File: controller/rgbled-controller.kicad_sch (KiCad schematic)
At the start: 23 parts, among them IC1 ME6211C33M5G-N, J1 PROG_HDR, J2 IC2_Header, J3 Power In, J4 Led Strip, J5 Power Selector, J6 3v3 Iin, Q1 UMH3N, Q2 2N7002, SW1 Reset, SW2 Flash, U1 ESP-12F

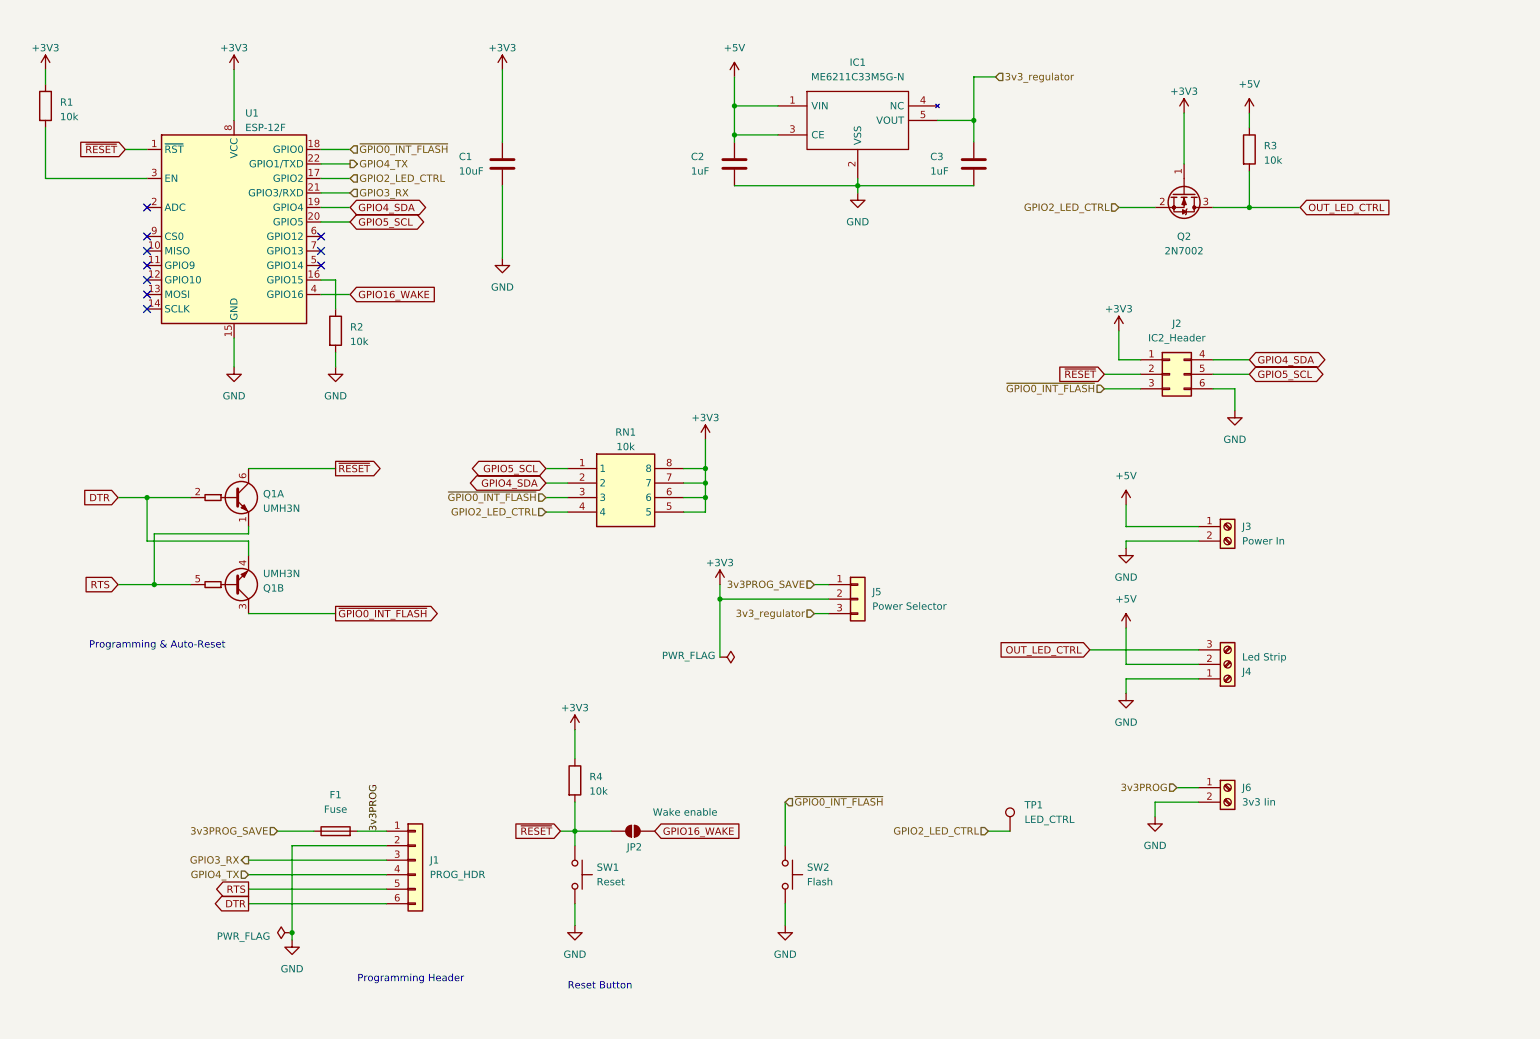
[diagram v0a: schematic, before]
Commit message: initial production version
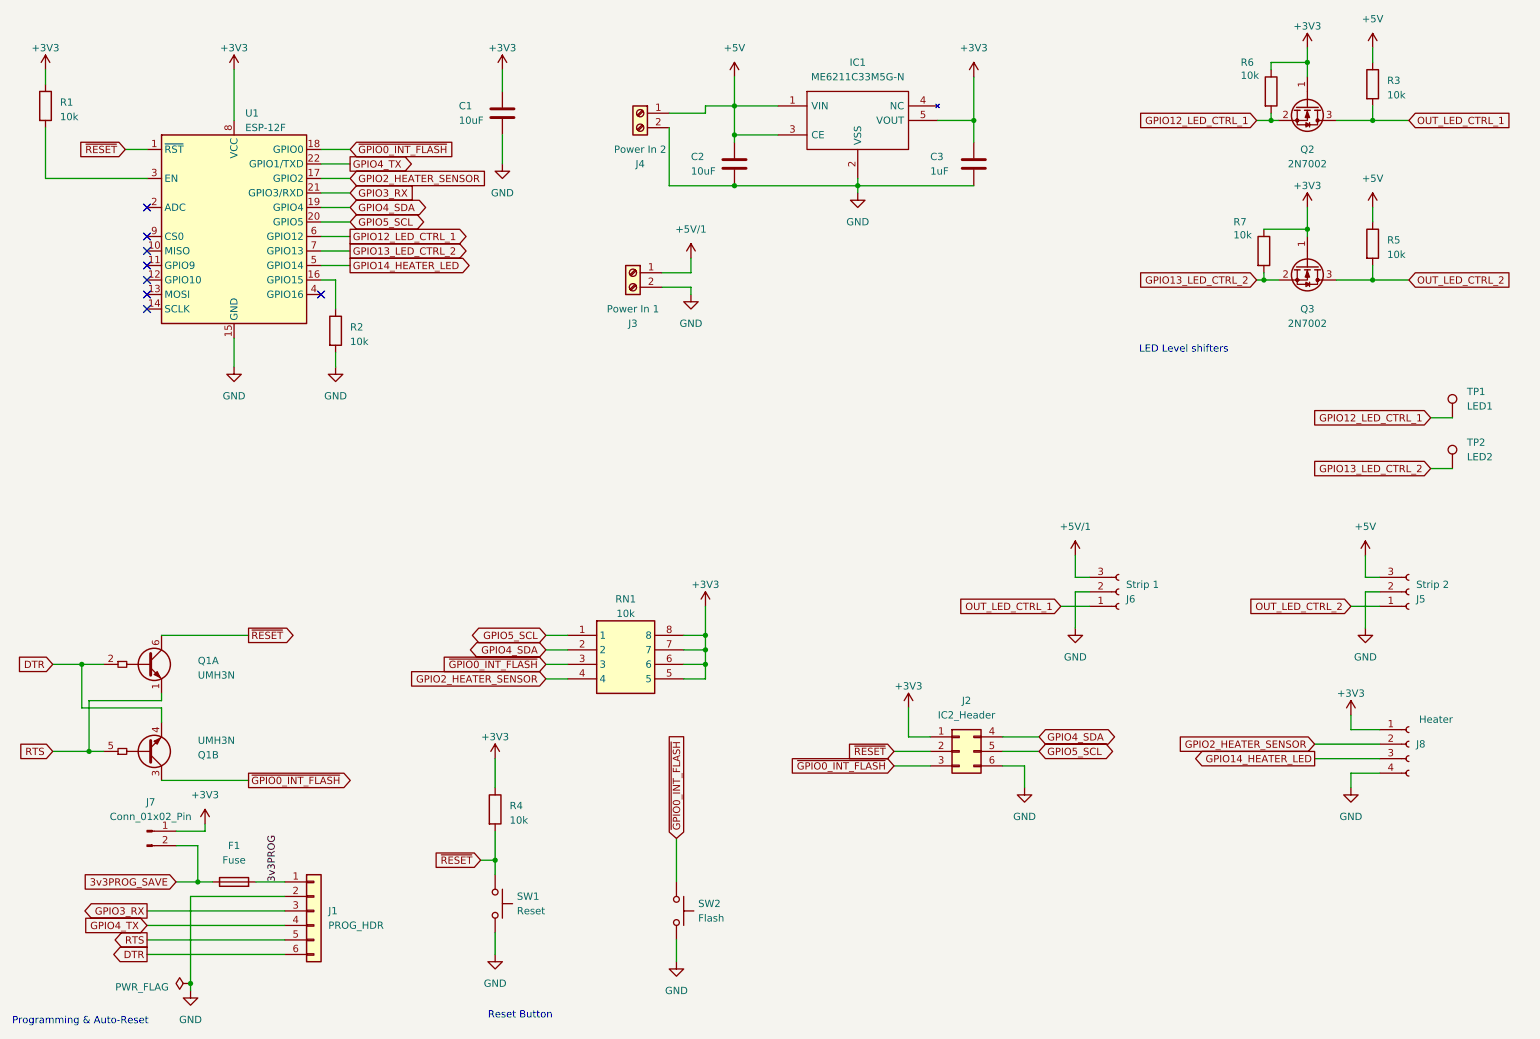
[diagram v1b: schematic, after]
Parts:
- removed J4: Led Strip, TerminalBlock:TerminalBlock_bornier-3_P5.08mm, symbol Connector:Screw_Terminal_01x03
- removed J5: Power Selector, Connector_PinHeader_2.54mm:PinHeader_1x03_P2.54mm_Vertical, symbol Connector_Generic:Conn_01x03
- removed J6: 3v3 Iin, TerminalBlock:TerminalBlock_bornier-2_P5.08mm, symbol Connector:Screw_Terminal_01x02
- removed JP2: Wake enable, Jumper:SolderJumper-2_P1.3mm_Open_Pad1.0x1.5mm, symbol Jumper:SolderJumper_2_Open
- added J4: Power In 2, TerminalBlock:TerminalBlock_bornier-2_P5.08mm, symbol Connector:Screw_Terminal_01x02
- added J5: Strip 2, TerminalBlock:TerminalBlock_bornier-3_P5.08mm, symbol Connector:Conn_01x03_Socket
- added J6: Strip 1, TerminalBlock:TerminalBlock_bornier-3_P5.08mm, symbol Connector:Conn_01x03_Socket
- added J7: Conn_01x02_Pin, Connector_PinHeader_2.54mm:PinHeader_1x02_P2.54mm_Vertical, symbol Connector:Conn_01x02_Pin
- added J8: Heater, Chof747_Connectors:CONN-TH_4P-P2.54_KF128-2.54-4P, symbol Connector:Conn_01x04_Socket
- added Q3: 2N7002, Package_TO_SOT_SMD:SOT-23, symbol Transistor_FET:2N7002
- added R5, R6, R7: 10k, Resistor_SMD:R_0603_1608Metric_Pad0.98x0.95mm_HandSolder, symbol Device:R
- added TP2: LED2, TestPoint:TestPoint_Pad_2.0x2.0mm, symbol Connector:TestPoint
- C2: value 1uF -> 10uF
- IC1: footprint SOT95P270X145-5N -> Chof747_Footprints:SOT95P270X145-5N
- J3: value Power In -> Power In 1
- RN1: footprint YC164JR07220RL -> Chof747_Footprints:YC164JR07220RL
- TP1: value LED_CTRL -> LED1
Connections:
- net 3v3_regulator is gone; now on net +3V3: C3.1, IC1.5 (VOUT)
- net +3V3: now also J7.1 (Pin_1), J8.1 (Pin_1), Q3.1 (G), R6.1, R7.1
- net +5V: now also J4.1 (Pin_1), J5.3 (Pin_3), R5.1; no longer J3.1 (Pin_1)
- net 3v3PROG_SAVE: now also J7.2 (Pin_2)
- net GND: now also J4.2 (Pin_2), J5.2 (Pin_2), J6.2 (Pin_2), J8.4 (Pin_4)
- net GPIO14_HEATER_LED: now reaches U1.5 (GPIO14)
- net GPIO14_HEATER_LED: now also J8.3 (Pin_3)
- net GPIO12_LED_CTRL_1: now reaches U1.6 (GPIO12)
- net GPIO12_LED_CTRL_1: now also Q2.2 (S), TP1.1, R6.2
- net GPIO13_LED_CTRL_2: now reaches U1.7 (GPIO13)
- net GPIO13_LED_CTRL_2: now also Q3.2 (S), R7.2, TP2.1
- net GPIO16_WAKE: no longer names the net of U1.4 (GPIO16)
- net GPIO2_LED_CTRL renamed GPIO2_HEATER_SENSOR
- net GPIO2_HEATER_SENSOR: now also J8.2 (Pin_2); no longer Q2.2 (S), TP1.1
- net OUT_LED_CTRL renamed OUT_LED_CTRL_1
- net OUT_LED_CTRL_1: now also J6.1 (Pin_1)
- new net +5V/1: J3.1 (Pin_1), J6.3 (Pin_3)
- new net OUT_LED_CTRL_2: J5.1 (Pin_1), Q3.3 (D), R5.2
- no-connect marks 10 -> 8
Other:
- note added: "LED Level shifters"
- note removed: "Programming Header"
- moved on the sheet: C1, F1, J1, J2, J3, Q1A, Q1B, Q2, R3, R4, RN1, SW1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
